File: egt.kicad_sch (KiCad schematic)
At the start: 9 parts, among them U4 MAX31855KASA

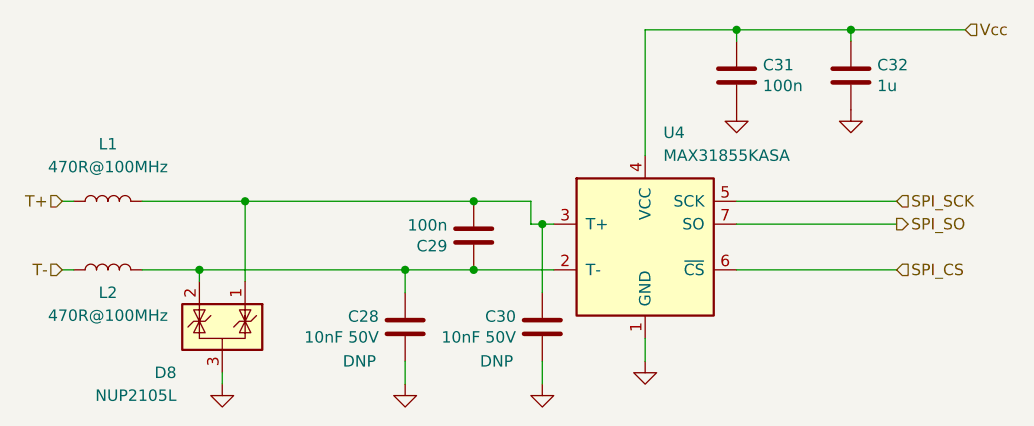
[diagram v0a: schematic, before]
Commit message: Placement
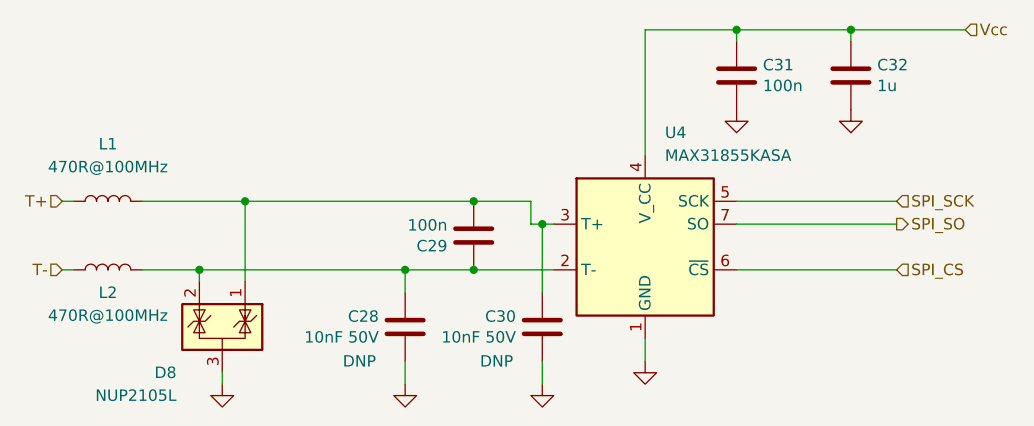
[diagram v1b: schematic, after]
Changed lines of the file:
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@@
     (effects (font (size 1.27 1.27)) (justify right))
   )
-  (symbol (lib_id "Device:C") (at 154.94 101.6 0) (mirror y) (unit 1)
-    (in_bom no) (on_board yes) (dnp no)
-    (property "Reference" "C30" (at 152.019 100.4316 0)
-      (effects (font (size 1.27 1.27)) (justify left))
-    )
-    (property "Value" "10nF 50V" (at 152.019 102.743 0)
-      (effects (font (size 1.27 1.27)) (justify left))
-    )
-    (property "Footprint" "Capacitor_SMD:C_0402_1005Metric" (at 153.9748 105.41 0)
-      (effects (font (size 1.27 1.27)) hide)
-    )
-    (property "Datasheet" "~" (at 154.94 101.6 0)
-      (effects (font (size 1.27 1.27)) hide)
-    )
-    (property "LCSC" "" (at 154.94 101.6 0)
-      (effects (font (size 1.27 1.27)) hide)
-    )
-    (property "MyComment" "DNP" (at 149.86 105.41 0)
-      (effects (font (size 1.27 1.27)))
-    )
-    (pin "1")
-    (pin "2")
-    (instances
-      (project "uaefi"
-        (path "/ac264c30-3e9a-4be2-b97a-9949b68bd497/ced20183-e5c8-42b4-80bd-35fc70d9313a"
-          (reference "C30") (unit 1)
-        )
-      )
-    )
-  )
-  (symbol (lib_id "Power_Protection:NUP2105L") (at 119.38 101.6 0) (mirror y) (unit 1)
-    (in_bom yes) (on_board yes) (dnp no)
-    (property "Reference" "D8" (at 114.3 106.68 0)
-      (effects (font (size 1.27 1.27)) (justify left))
-    )
-    (property "Value" "NUP2105L" (at 114.3 109.22 0)
-      (effects (font (size 1.27 1.27)) (justify left))
-    )
-    (property "Footprint" "Package_TO_SOT_SMD:SOT-23" (at 113.665 102.87 0)
-      (effects (font (size 1.27 1.27)) (justify left) hide)
-    )
-    (property "Datasheet" "http://www.onsemi.com/pub_link/Collateral/NUP2105L-D.PDF" (at 116.205 98.425 0)
-      (effects (font (size 1.27 1.27)) hide)
-    )
-    (property "LCSC" "C284104" (at 119.38 101.6 0)
-      (effects (font (size 1.27 1.27)) hide)
-    )
-    (pin "3")
-    (pin "1")
-    (pin "2")
-    (instances
-      (project "uaefi"
-        (path "/ac264c30-3e9a-4be2-b97a-9949b68bd497/ced20183-e5c8-42b4-80bd-35fc70d9313a"
-          (reference "D8") (unit 1)
-        )
-      )
-    )
-  )
-  (symbol (lib_id "Sensor_Temperature:MAX31855KASA") (at 166.37 92.71 0) (unit 1)
+  (symbol (lib_name "MAX31855KASA_1") (lib_id "Sensor_Temperature:MAX31855KASA") (at 166.37 92.71 0) (unit 1)
     (in_bom yes) (on_board yes) (dnp no) (fields_autoplaced)
-    (property "Reference" "U4" (at 168.3894 80.01 0)
-      (effects (font (size 1.27 1.27)) (justify left))
-    )
-    (property "Value" "MAX31855KASA" (at 168.3894 82.55 0)
+    (property "Reference" "U4" (at 168.5641 80.01 0)
+      (effects (font (size 1.27 1.27)) (justify left))
+    )
+    (property "Value" "MAX31855KASA" (at 168.5641 82.55 0)
       (effects (font (size 1.27 1.27)) (justify left))
     )
@@
     )
   )
+  (symbol (lib_id "Device:C") (at 154.94 101.6 0) (mirror y) (unit 1)
+    (in_bom no) (on_board yes) (dnp no)
+    (property "Reference" "C30" (at 152.019 100.4316 0)
+      (effects (font (size 1.27 1.27)) (justify left))
+    )
+    (property "Value" "10nF 50V" (at 152.019 102.743 0)
+      (effects (font (size 1.27 1.27)) (justify left))
+    )
+    (property "Footprint" "Capacitor_SMD:C_0402_1005Metric" (at 153.9748 105.41 0)
+      (effects (font (size 1.27 1.27)) hide)
+    )
+    (property "Datasheet" "~" (at 154.94 101.6 0)
+      (effects (font (size 1.27 1.27)) hide)
+    )
+    (property "LCSC" "" (at 154.94 101.6 0)
+      (effects (font (size 1.27 1.27)) hide)
+    )
+    (property "MyComment" "DNP" (at 149.86 105.41 0)
+      (effects (font (size 1.27 1.27)))
+    )
+    (pin "1")
+    (pin "2")
+    (instances
+      (project "uaefi"
+        (path "/ac264c30-3e9a-4be2-b97a-9949b68bd497/ced20183-e5c8-42b4-80bd-35fc70d9313a"
+          (reference "C30") (unit 1)
+        )
+      )
+    )
+  )
+  (symbol (lib_id "Power_Protection:NUP2105L") (at 119.38 101.6 0) (mirror y) (unit 1)
+    (in_bom yes) (on_board yes) (dnp no)
+    (property "Reference" "D8" (at 114.3 106.68 0)
+      (effects (font (size 1.27 1.27)) (justify left))
+    )
+    (property "Value" "NUP2105L" (at 114.3 109.22 0)
+      (effects (font (size 1.27 1.27)) (justify left))
+    )
+    (property "Footprint" "Package_TO_SOT_SMD:SOT-23" (at 113.665 102.87 0)
+      (effects (font (size 1.27 1.27)) (justify left) hide)
+    )
+    (property "Datasheet" "http://www.onsemi.com/pub_link/Collateral/NUP2105L-D.PDF" (at 116.205 98.425 0)
+      (effects (font (size 1.27 1.27)) hide)
+    )
+    (property "LCSC" "C284104" (at 119.38 101.6 0)
+      (effects (font (size 1.27 1.27)) hide)
+    )
+    (pin "3")
+    (pin "1")
+    (pin "2")
+    (instances
+      (project "uaefi"
+        (path "/ac264c30-3e9a-4be2-b97a-9949b68bd497/ced20183-e5c8-42b4-80bd-35fc70d9313a"
+          (reference "D8") (unit 1)
+        )
+      )
+    )
+  )
   (symbol (lib_id "Device:L") (at 106.68 87.63 90) (unit 1)
     (in_bom yes) (on_board yes) (dnp no)
@@
     )
   )
-  (symbol (lib_name "GND_4") (lib_id "power:GND") (at 176.53 77.47 0) (unit 1)
+  (symbol (lib_id "power:GND") (at 176.53 77.47 0) (unit 1)
     (in_bom yes) (on_board yes) (dnp no)
     (property "Reference" "#PWR0109" (at 176.53 83.82 0)
@@
     )
   )
-  (symbol (lib_name "GND_3") (lib_id "power:GND") (at 189.23 77.47 0) (unit 1)
+  (symbol (lib_id "power:GND") (at 189.23 77.47 0) (unit 1)
     (in_bom yes) (on_board yes) (dnp no)
     (property "Reference" "#PWR0110" (at 189.23 83.82 0)
@@
     )
   )
-  (symbol (lib_name "GND_5") (lib_id "power:GND") (at 139.7 107.95 0) (unit 1)
+  (symbol (lib_id "power:GND") (at 139.7 107.95 0) (unit 1)
     (in_bom yes) (on_board yes) (dnp no)
     (property "Reference" "#PWR0106" (at 139.7 114.3 0)
@@
     )
   )
-  (symbol (lib_name "GND_6") (lib_id "power:GND") (at 154.94 107.95 0) (unit 1)
+  (symbol (lib_id "power:GND") (at 154.94 107.95 0) (unit 1)
     (in_bom yes) (on_board yes) (dnp no)
     (property "Reference" "#PWR0107" (at 154.94 114.3 0)
@@
     )
   )
-  (symbol (lib_name "GND_7") (lib_id "power:GND") (at 166.37 105.41 0) (unit 1)
+  (symbol (lib_id "power:GND") (at 166.37 105.41 0) (unit 1)
     (in_bom yes) (on_board yes) (dnp no)
     (property "Reference" "#PWR0108" (at 166.37 111.76 0)
